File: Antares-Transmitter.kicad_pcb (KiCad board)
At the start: 2 copper layers, 94 x 60.8 mm, 99 parts, among them J1001 Debugger Pin, J1101 Conn_01x02, J401 Conn_01x11, J501 Conn_01x03, J601 Conn_01x05, J602 Conn_01x06, J901 Conn_01x05, SW701 DOWN, SW702 UP, U201 STM32G070KBTx, U301 CC1101RGPR, U401 74HC165, U402 74HC165, U801 LIS3DHTR, Y301 27MHz

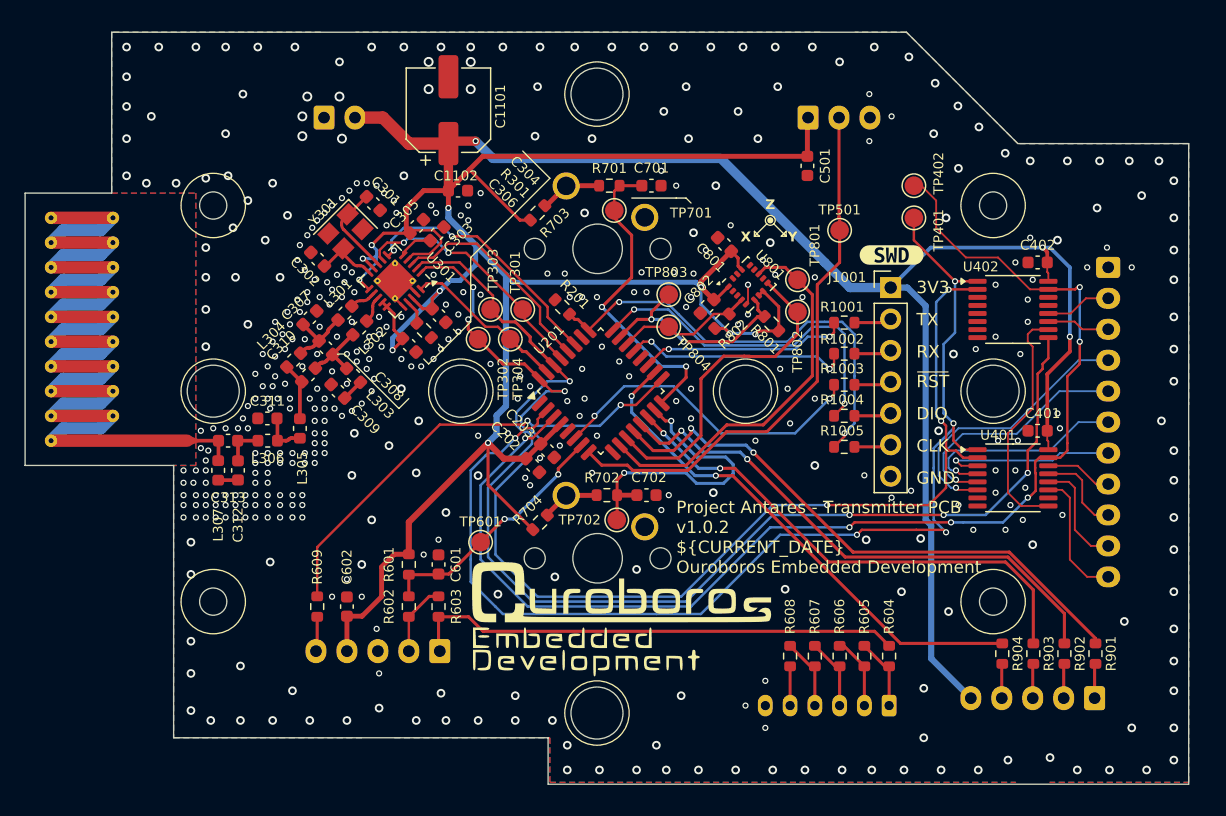
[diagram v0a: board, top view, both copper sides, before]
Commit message: small fixes
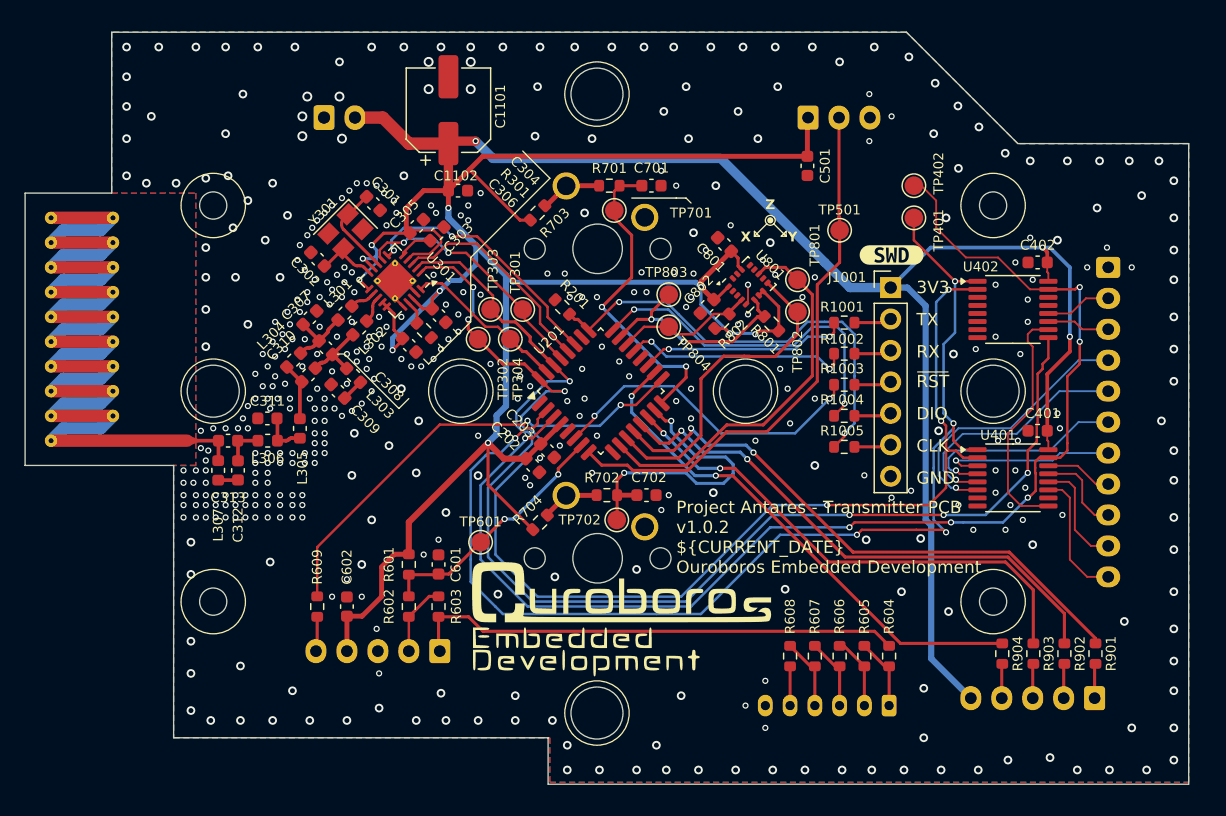
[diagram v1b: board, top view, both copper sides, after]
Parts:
- J1101: footprint Connector_JST:JST_XA_S02B-XASK-1_1x02_P2.50mm_Horizontal -> Connector_JST:JST_XH_S2B-XH-A-1_1x02_P2.50mm_Horizontal
- J401: footprint Connector_JST:JST_XA_S11B-XASK-1_1x11_P2.50mm_Horizontal -> Connector_JST:JST_XH_S11B-XH-A-1_1x11_P2.50mm_Horizontal
- J501: footprint Connector_JST:JST_XA_S03B-XASK-1_1x03_P2.50mm_Horizontal -> Connector_JST:JST_XH_S3B-XH-A-1_1x03_P2.50mm_Horizontal
- J601, J901: footprint Connector_JST:JST_XA_S05B-XASK-1_1x05_P2.50mm_Horizontal -> Connector_JST:JST_XH_S5B-XH-A-1_1x05_P2.50mm_Horizontal
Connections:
- U402 pad 9: /Notes/HC165_DO -> Net-(U402-Q7)
